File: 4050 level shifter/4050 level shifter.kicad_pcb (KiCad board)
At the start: 2 copper layers, 73.7 x 50.8 mm, 16 parts, among them J1 Conn_01x03, J10 In, J11 Out, J12 In, J13 Out, J14 5V, J15 GND, J2 In, J3 Out, J4 In, J5 Out, J6 In, J7 Out, J8 In, J9 Out, U1 4050

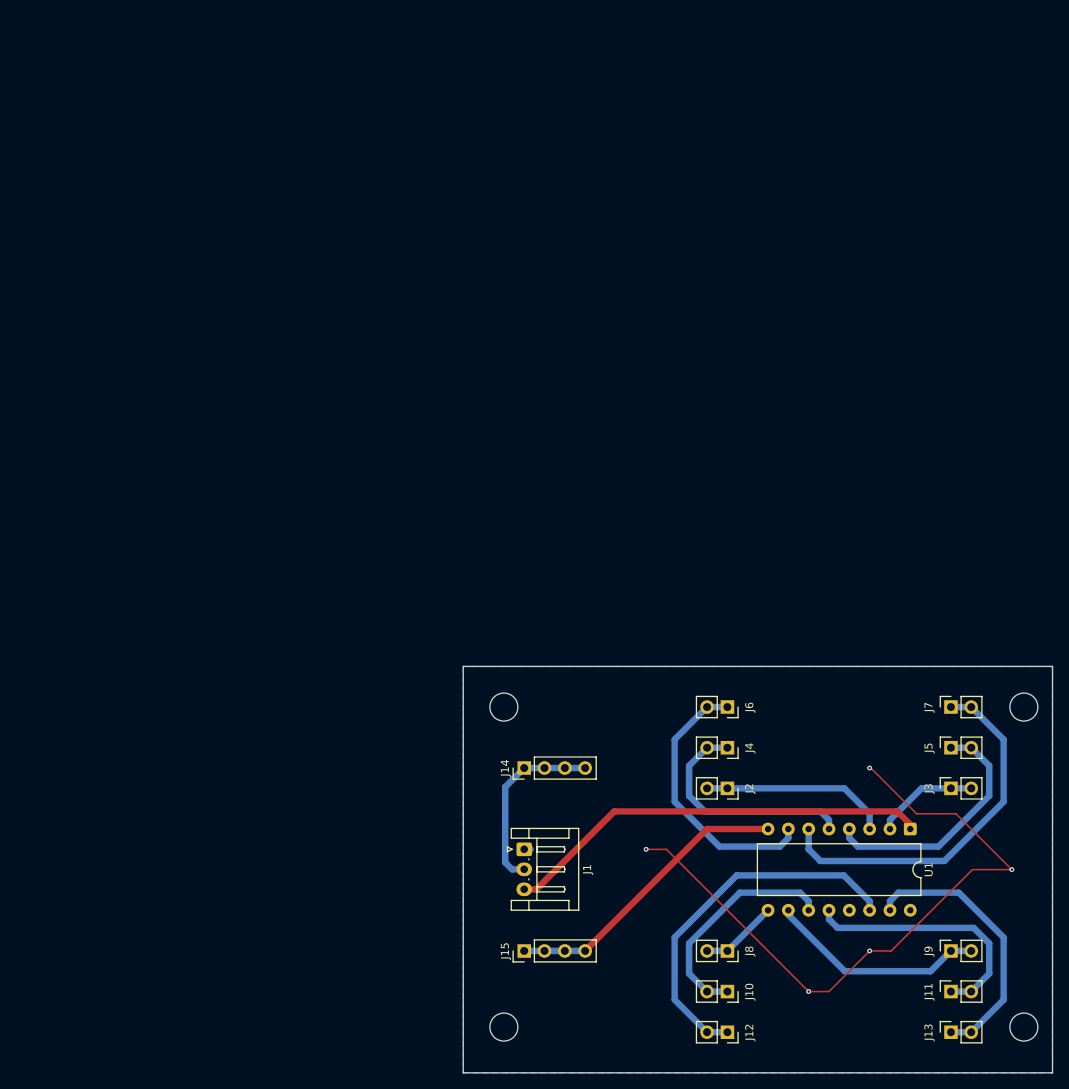
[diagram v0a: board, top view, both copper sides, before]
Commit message: more change in gerbers
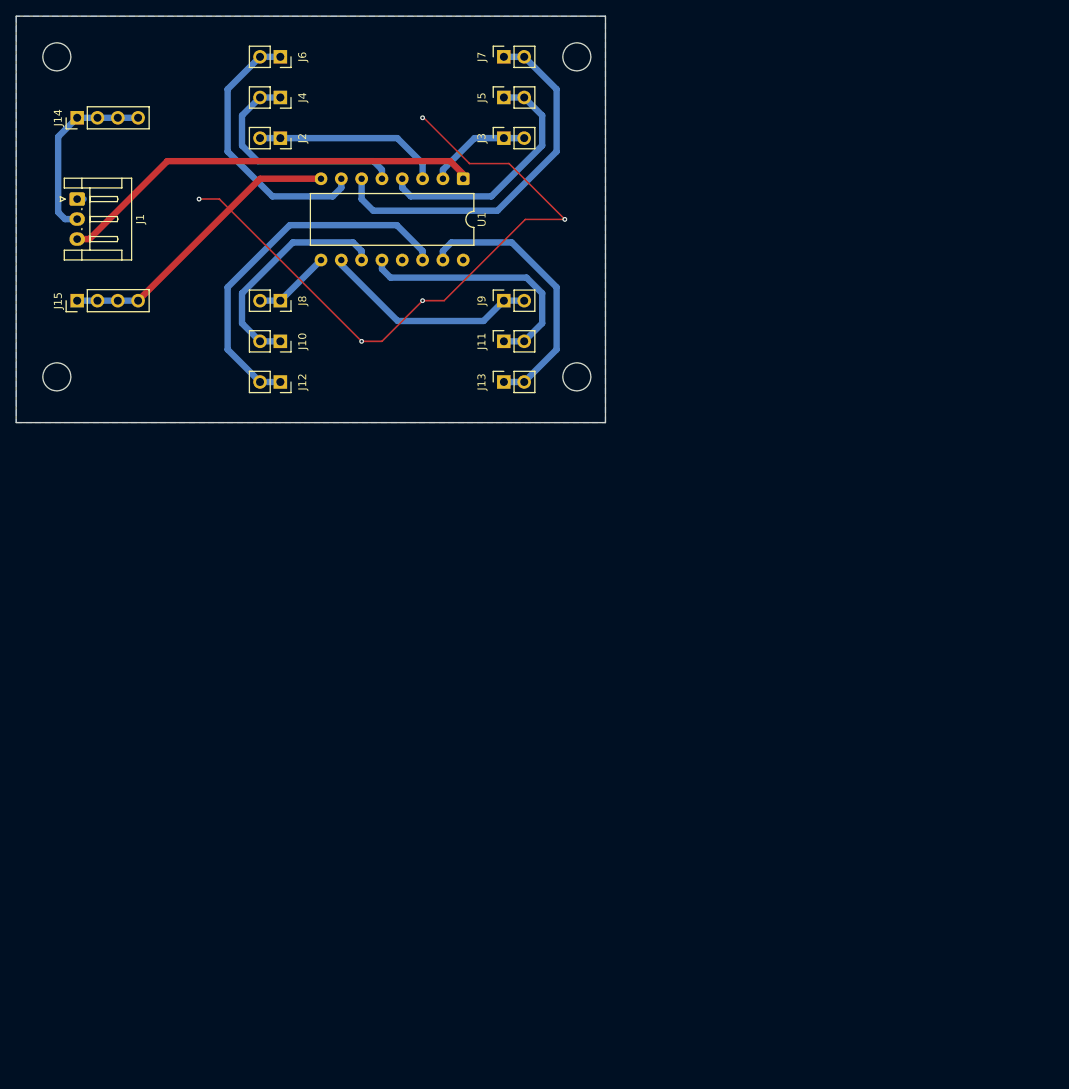
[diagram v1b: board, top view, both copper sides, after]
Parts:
- moved J1 98.6 mm to (7.62, 22.9)
- moved J10 98.6 mm to (33.0, 40.6)
- moved J11 98.6 mm to (61.0, 40.6)
- moved J12 98.6 mm to (33.0, 45.7)
- moved J13 98.6 mm to (61.0, 45.7)
- moved J14 98.6 mm to (7.62, 12.7)
- moved J15 98.6 mm to (7.62, 35.6)
- moved J2 98.6 mm to (33.0, 15.2)
- moved J3 98.6 mm to (61.0, 15.2)
- moved J4 98.6 mm to (33.0, 10.2)
- moved J5 98.6 mm to (61.0, 10.2)
- moved J6 98.6 mm to (33.0, 5.08)
- moved J7 98.6 mm to (61.0, 5.08)
- moved J8 98.6 mm to (33.0, 35.6)
- moved J9 98.6 mm to (61.0, 35.6)
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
